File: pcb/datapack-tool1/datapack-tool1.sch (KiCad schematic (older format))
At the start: 4 parts

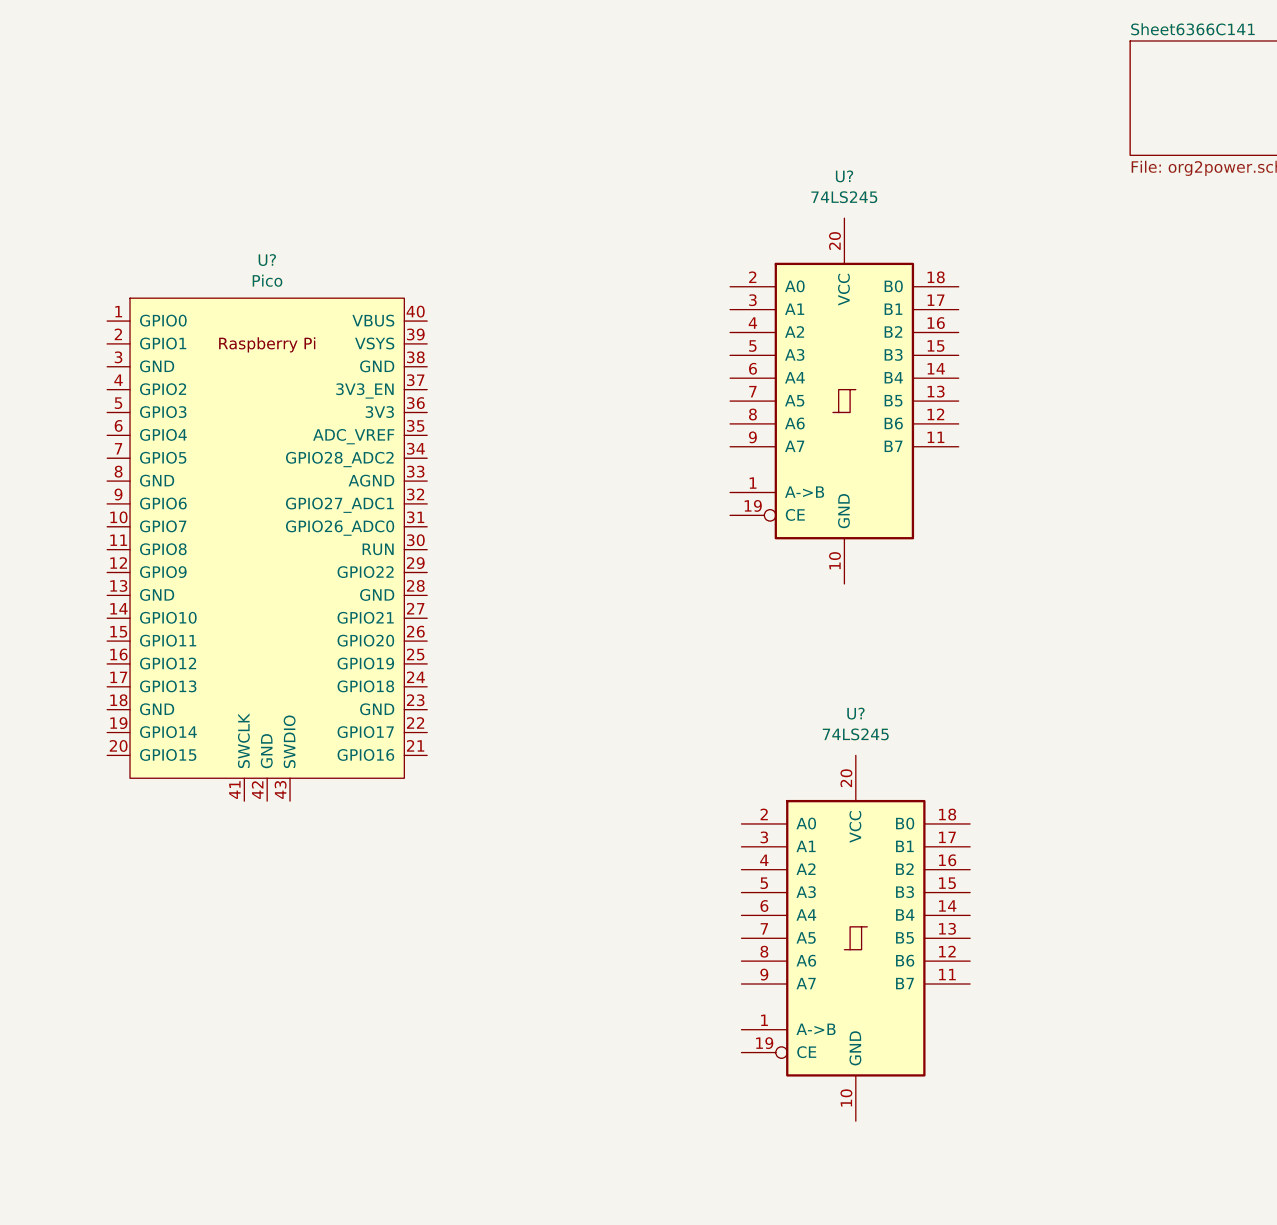
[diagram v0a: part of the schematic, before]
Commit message: Updates
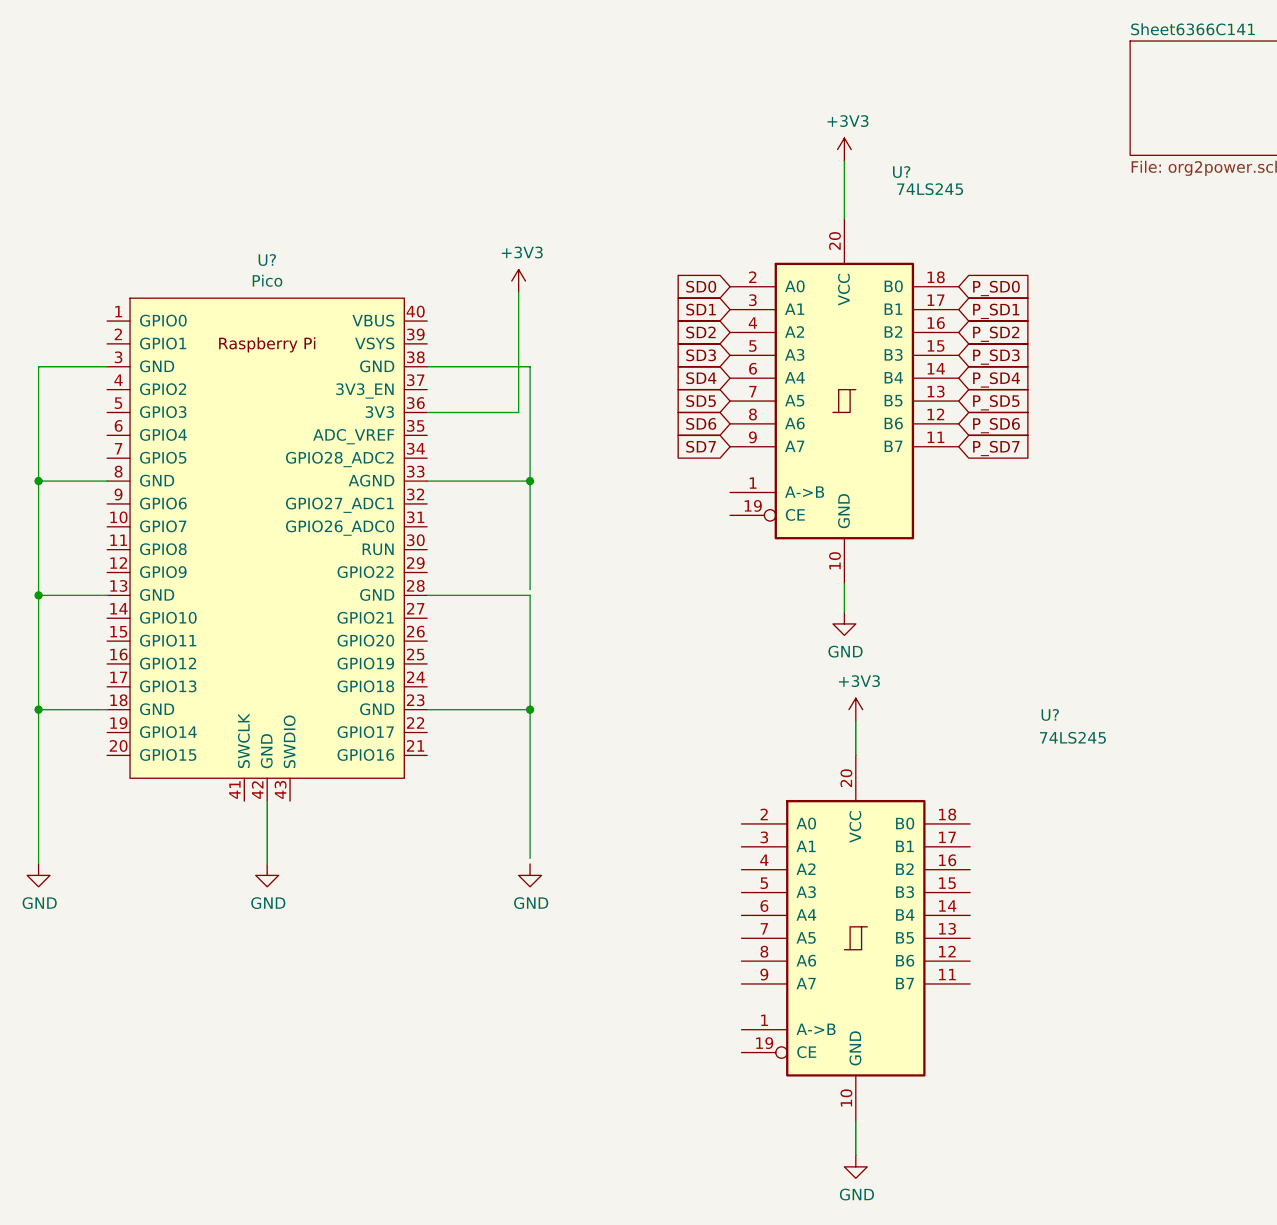
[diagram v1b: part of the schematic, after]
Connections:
- net labels added: +3V3, SD0, SD1, SD2, SD3, SD4, SD5, SD6, SD7
- wire segments 3 -> 26
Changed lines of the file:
@@
 U 1 1 63677927
 P 4850 2325
-F 0 "U?" H 4850 3306 50  0000 C CNN
-F 1 "74LS245" H 4850 3215 50  0000 C CNN
+F 0 "U?" H 5100 3325 50  0000 C CNN
+F 1 "74LS245" H 5225 3250 50  0000 C CNN
 F 2 "" H 4850 2325 50  0001 C CNN
 F 3 "http://www.ti.com/lit/gpn/sn74LS245" H 4850 2325 50  0001 C CNN
@@
 U 1 1 63678AE8
 P 4900 4675
-F 0 "U?" H 4900 5656 50  0000 C CNN
-F 1 "74LS245" H 4900 5565 50  0000 C CNN
+F 0 "U?" H 5750 5650 50  0000 C CNN
+F 1 "74LS245" H 5850 5550 50  0000 C CNN
 F 2 "" H 4900 4675 50  0001 C CNN
 F 3 "http://www.ti.com/lit/gpn/sn74LS245" H 4900 4675 50  0001 C CNN
@@
 	1    0    0    -1
 $EndComp
+$Comp
+L power:GND #PWR?
+U 1 1 6367C304
+P 2325 4350
+F 0 "#PWR?" H 2325 4100 50  0001 C CNN
+F 1 "GND" H 2330 4177 50  0000 C CNN
+F 2 "" H 2325 4350 50  0001 C CNN
+F 3 "" H 2325 4350 50  0001 C CNN
+	1    2325 4350
+	1    0    0    -1
+$EndComp
+$Comp
+L power:GND #PWR?
+U 1 1 6367C6EB
+P 4850 3250
+F 0 "#PWR?" H 4850 3000 50  0001 C CNN
+F 1 "GND" H 4855 3077 50  0000 C CNN
+F 2 "" H 4850 3250 50  0001 C CNN
+F 3 "" H 4850 3250 50  0001 C CNN
+	1    4850 3250
+	1    0    0    -1
+$EndComp
+$Comp
+L power:GND #PWR?
+U 1 1 6367CA98
+P 4900 5625
+F 0 "#PWR?" H 4900 5375 50  0001 C CNN
+F 1 "GND" H 4905 5452 50  0000 C CNN
+F 2 "" H 4900 5625 50  0001 C CNN
+F 3 "" H 4900 5625 50  0001 C CNN
+	1    4900 5625
+	1    0    0    -1
+$EndComp
+$Comp
+L power:+3V3 #PWR?
+U 1 1 6367D4B6
+P 3425 1850
+F 0 "#PWR?" H 3425 1700 50  0001 C CNN
+F 1 "+3V3" H 3440 2023 50  0000 C CNN
+F 2 "" H 3425 1850 50  0001 C CNN
+F 3 "" H 3425 1850 50  0001 C CNN
+	1    3425 1850
+	1    0    0    -1
+$EndComp
+$Comp
+L power:+3V3 #PWR?
+U 1 1 6367D50D
+P 4900 3725
+F 0 "#PWR?" H 4900 3575 50  0001 C CNN
+F 1 "+3V3" H 4915 3898 50  0000 C CNN
+F 2 "" H 4900 3725 50  0001 C CNN
+F 3 "" H 4900 3725 50  0001 C CNN
+	1    4900 3725
+	1    0    0    -1
+$EndComp
+$Comp
+L power:+3V3 #PWR?
+U 1 1 6367D984
+P 4850 1275
+F 0 "#PWR?" H 4850 1125 50  0001 C CNN
+F 1 "+3V3" H 4865 1448 50  0000 C CNN
+F 2 "" H 4850 1275 50  0001 C CNN
+F 3 "" H 4850 1275 50  0001 C CNN
+	1    4850 1275
+	1    0    0    -1
+$EndComp
+Wire Wire Line
+	4850 1275 4850 1525
+Wire Wire Line
+	3425 1850 3425 2375
+Wire Wire Line
+	3425 2375 3025 2375
+Wire Wire Line
+	4850 3125 4850 3250
+Wire Wire Line
+	4900 5475 4900 5625
+Wire Wire Line
+	4900 3725 4900 3875
+Wire Wire Line
+	2325 4075 2325 4350
+$Comp
+L power:GND #PWR?
+U 1 1 63680DDA
+P 1325 4350
+F 0 "#PWR?" H 1325 4100 50  0001 C CNN
+F 1 "GND" H 1330 4177 50  0000 C CNN
+F 2 "" H 1325 4350 50  0001 C CNN
+F 3 "" H 1325 4350 50  0001 C CNN
+	1    1325 4350
+	1    0    0    -1
+$EndComp
+$Comp
+L power:GND #PWR?
+U 1 1 6368129A
+P 3475 4350
+F 0 "#PWR?" H 3475 4100 50  0001 C CNN
+F 1 "GND" H 3480 4177 50  0000 C CNN
+F 2 "" H 3475 4350 50  0001 C CNN
+F 3 "" H 3475 4350 50  0001 C CNN
+	1    3475 4350
+	1    0    0    -1
+$EndComp
+Wire Wire Line
+	1325 4350 1325 3675
+Wire Wire Line
+	1325 3675 1625 3675
+Wire Wire Line
+	1625 3175 1325 3175
+Wire Wire Line
+	1325 3175 1325 3675
+Connection ~ 1325 3675
+Wire Wire Line
+	3475 4325 3475 3675
+Wire Wire Line
+	3475 3675 3025 3675
+Wire Wire Line
+	3475 3675 3475 3175
+Wire Wire Line
+	3475 3175 3025 3175
+Connection ~ 3475 3675
+Wire Wire Line
+	3475 3150 3475 2675
+Wire Wire Line
+	3475 2675 3025 2675
+Wire Wire Line
+	1325 3175 1325 2675
+Wire Wire Line
+	1325 2675 1625 2675
+Connection ~ 1325 3175
+Wire Wire Line
+	1625 2175 1325 2175
+Wire Wire Line
+	1325 2175 1325 2675
+Connection ~ 1325 2675
+Wire Wire Line
+	3025 2175 3475 2175
+Wire Wire Line
+	3475 2175 3475 2675
+Connection ~ 3475 2675
+Text GLabel 5350 1825 2    50   Input ~ 0
+P_SD0
+Text GLabel 5350 1925 2    50   Input ~ 0
+P_SD1
+Text GLabel 5350 2025 2    50   Input ~ 0
+P_SD2
+Text GLabel 5350 2125 2    50   Input ~ 0
+P_SD3
+Text GLabel 5350 2225 2    50   Input ~ 0
+P_SD4
+Text GLabel 5350 2325 2    50   Input ~ 0
+P_SD5
+Text GLabel 5350 2425 2    50   Input ~ 0
+P_SD6
+Text GLabel 5350 2525 2    50   Input ~ 0
+P_SD7
+Text GLabel 4350 1825 0    50   Input ~ 0
+SD0
+Text GLabel 4350 1925 0    50   Input ~ 0
+SD1
+Text GLabel 4350 2025 0    50   Input ~ 0
+SD2
+Text GLabel 4350 2125 0    50   Input ~ 0
+SD3
+Text GLabel 4350 2225 0    50   Input ~ 0
+SD4
+Text GLabel 4350 2325 0    50   Input ~ 0
+SD5
+Text GLabel 4350 2425 0    50   Input ~ 0
+SD6
+Text GLabel 4350 2525 0    50   Input ~ 0
+SD7
 $EndSCHEMATC

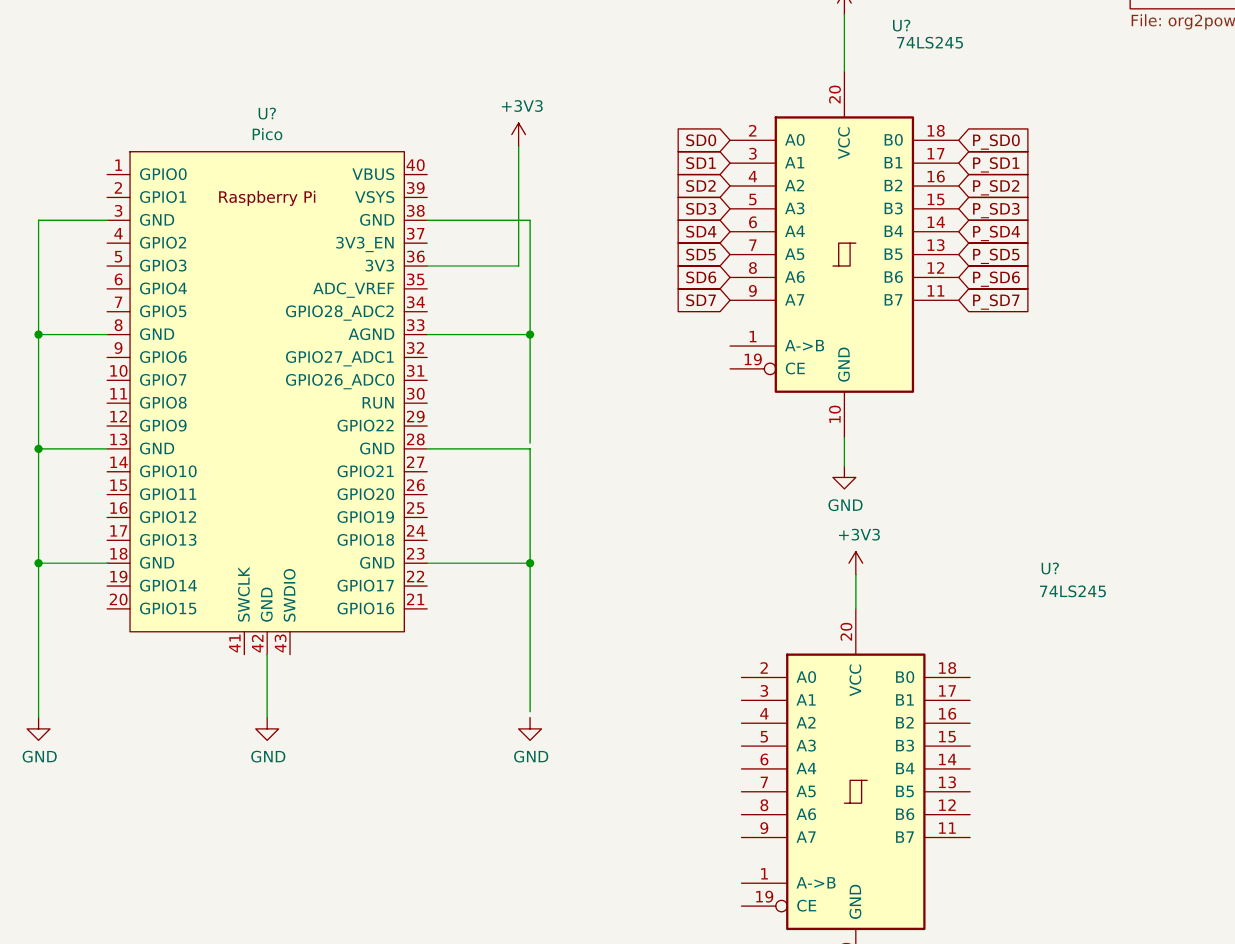
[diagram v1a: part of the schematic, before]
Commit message: Updates
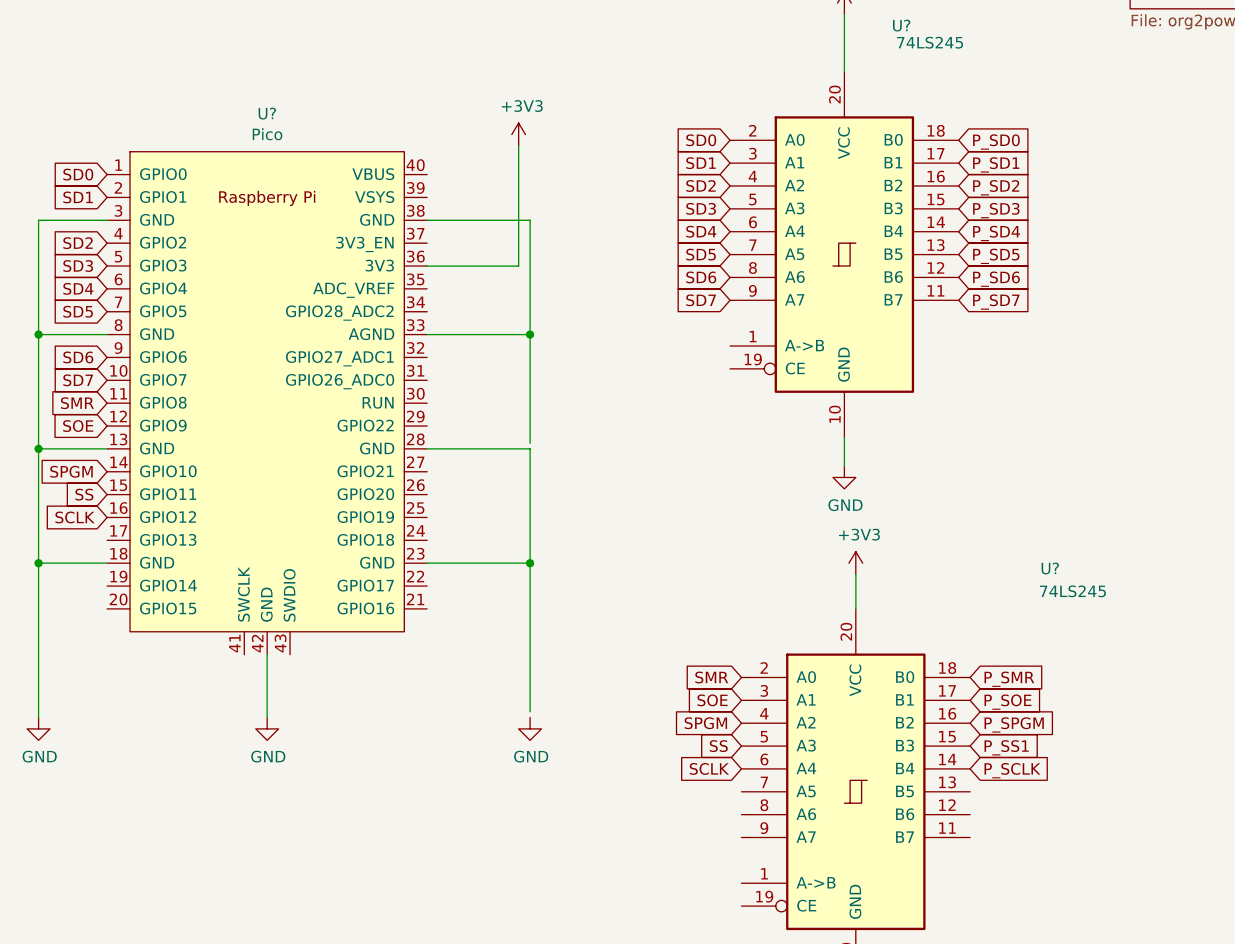
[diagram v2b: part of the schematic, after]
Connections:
- net labels added: SCLK, SMR, SOE, SPGM, SS
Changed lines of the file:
@@
 Text GLabel 4350 2525 0    50   Input ~ 0
 SD7
+Text GLabel 1625 1975 0    50   Input ~ 0
+SD0
+Text GLabel 1625 2075 0    50   Input ~ 0
+SD1
+Text GLabel 1625 2275 0    50   Input ~ 0
+SD2
+Text GLabel 1625 2375 0    50   Input ~ 0
+SD3
+Text GLabel 1625 2475 0    50   Input ~ 0
+SD4
+Text GLabel 1625 2575 0    50   Input ~ 0
+SD5
+Text GLabel 1625 2775 0    50   Input ~ 0
+SD6
+Text GLabel 1625 2875 0    50   Input ~ 0
+SD7
+Text GLabel 5400 4175 2    50   Input ~ 0
+P_SMR
+Text GLabel 5400 4275 2    50   Input ~ 0
+P_SOE
+Text GLabel 5400 4575 2    50   Input ~ 0
+P_SCLK
+Text GLabel 5400 4475 2    50   Input ~ 0
+P_SS1
+Text GLabel 5400 4375 2    50   Input ~ 0
+P_SPGM
+Text GLabel 4400 4175 0    50   Input ~ 0
+SMR
+Text GLabel 4400 4275 0    50   Input ~ 0
+SOE
+Text GLabel 4400 4375 0    50   Input ~ 0
+SPGM
+Text GLabel 4400 4475 0    50   Input ~ 0
+SS
+Text GLabel 4400 4575 0    50   Input ~ 0
+SCLK
+Text GLabel 1625 2975 0    50   Input ~ 0
+SMR
+Text GLabel 1625 3075 0    50   Input ~ 0
+SOE
+Text GLabel 1625 3275 0    50   Input ~ 0
+SPGM
+Text GLabel 1625 3375 0    50   Input ~ 0
+SS
+Text GLabel 1625 3475 0    50   Input ~ 0
+SCLK
 $EndSCHEMATC
